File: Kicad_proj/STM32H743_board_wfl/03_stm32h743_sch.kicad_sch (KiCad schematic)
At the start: 1 part, among them U1 STM32H743VITx

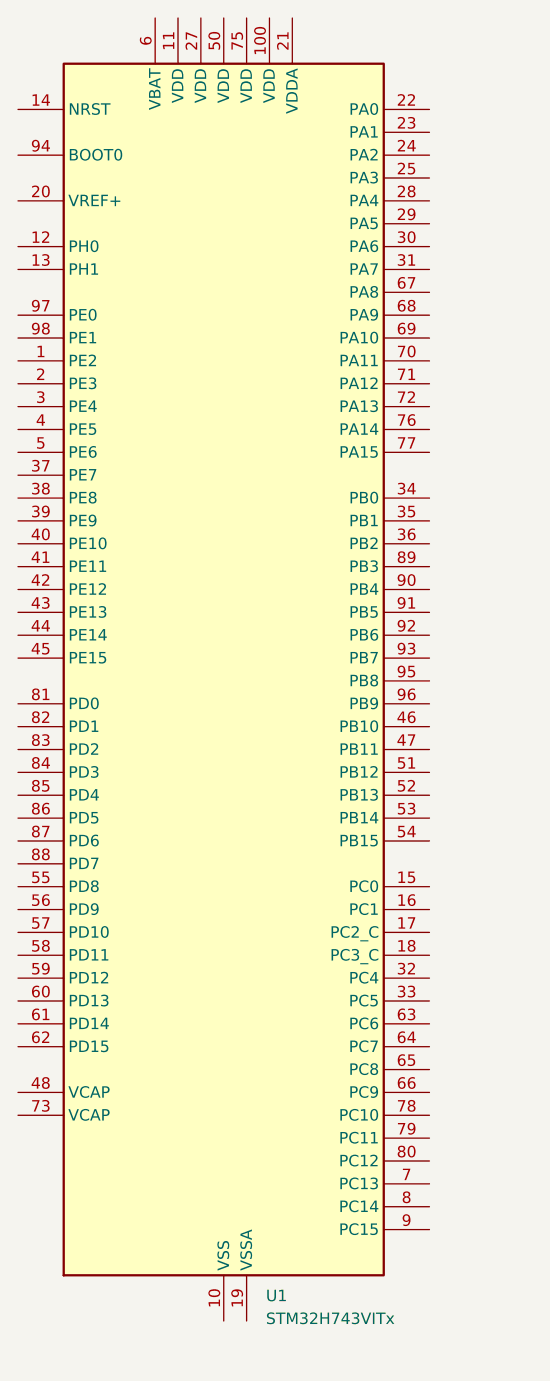
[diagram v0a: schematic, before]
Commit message: v0.3 uzupelniony prebom + placement BMI088 na sch
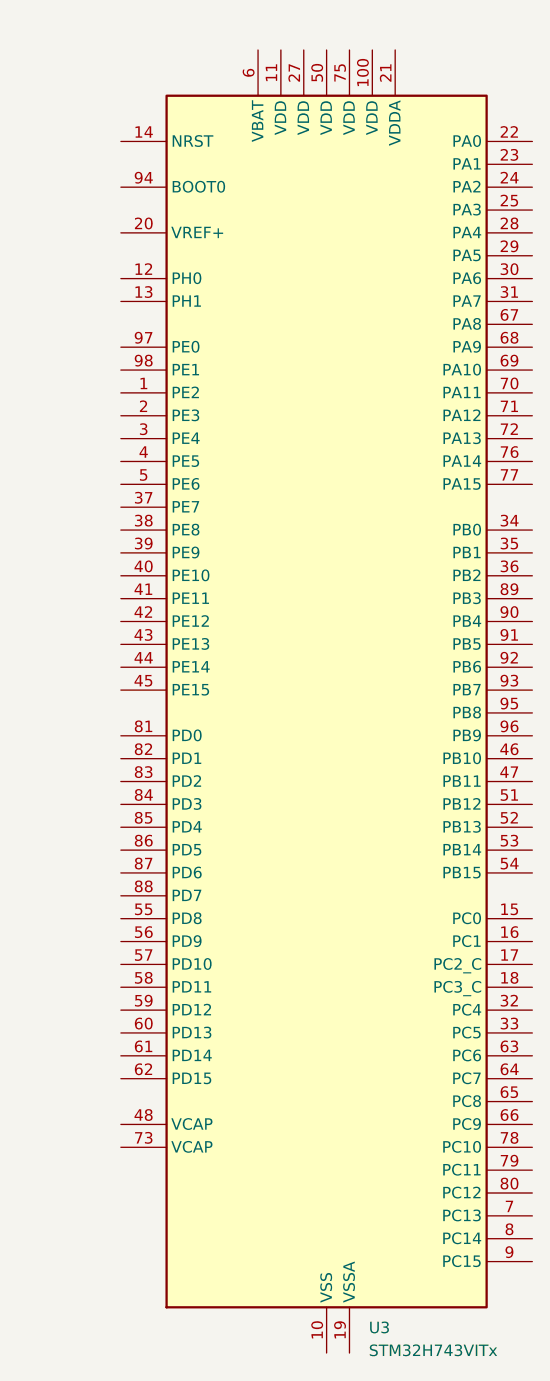
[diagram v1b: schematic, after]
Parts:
- renumbered U1 to U3
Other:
- moved on the sheet: U3
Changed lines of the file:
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@@
 	(symbol
 		(lib_id "MCU_ST_STM32H7:STM32H743VITx")
-		(at 214.884 132.588 0)
+		(at 226.314 136.144 0)
 		(unit 1)
 		(body_style 1)
@@
 		(dnp no)
 		(fields_autoplaced yes)
-		(property "Reference" "U1"
-			(at 219.5673 200.914 0)
+		(property "Reference" "U3"
+			(at 230.9973 204.47 0)
 			(show_name no)
 			(do_not_autoplace no)
@@
 		)
 		(property "Value" "STM32H743VITx"
-			(at 219.5673 203.454 0)
+			(at 230.9973 207.01 0)
 			(show_name no)
 			(do_not_autoplace no)
@@
 		)
 		(property "Footprint" "Package_QFP:LQFP-100_14x14mm_P0.5mm"
-			(at 197.104 198.628 0)
+			(at 208.534 202.184 0)
 			(hide yes)
 			(show_name no)
@@
 		)
 		(property "Datasheet" "https://www.st.com/resource/en/datasheet/stm32h743vi.pdf"
-			(at 214.884 132.588 0)
+			(at 226.314 136.144 0)
 			(hide yes)
 			(show_name no)
@@
 		)
 		(property "Description" "STMicroelectronics Arm Cortex-M7 MCU, 2048KB flash, 1024KB RAM, 480 MHz, 1.71-3.6V, 82 GPIO, LQFP100"
-			(at 214.884 132.588 0)
+			(at 226.314 136.144 0)
 			(hide yes)
 			(show_name no)
@@
 			(project "STM32H743_board_wfl"
 				(path "/3ffbaf01-8fe7-4f96-b685-21b9df9d548a/d99da23c-42db-4338-87a0-b38c4540e099"
-					(reference "U1")
+					(reference "U3")
 					(unit 1)
 				)

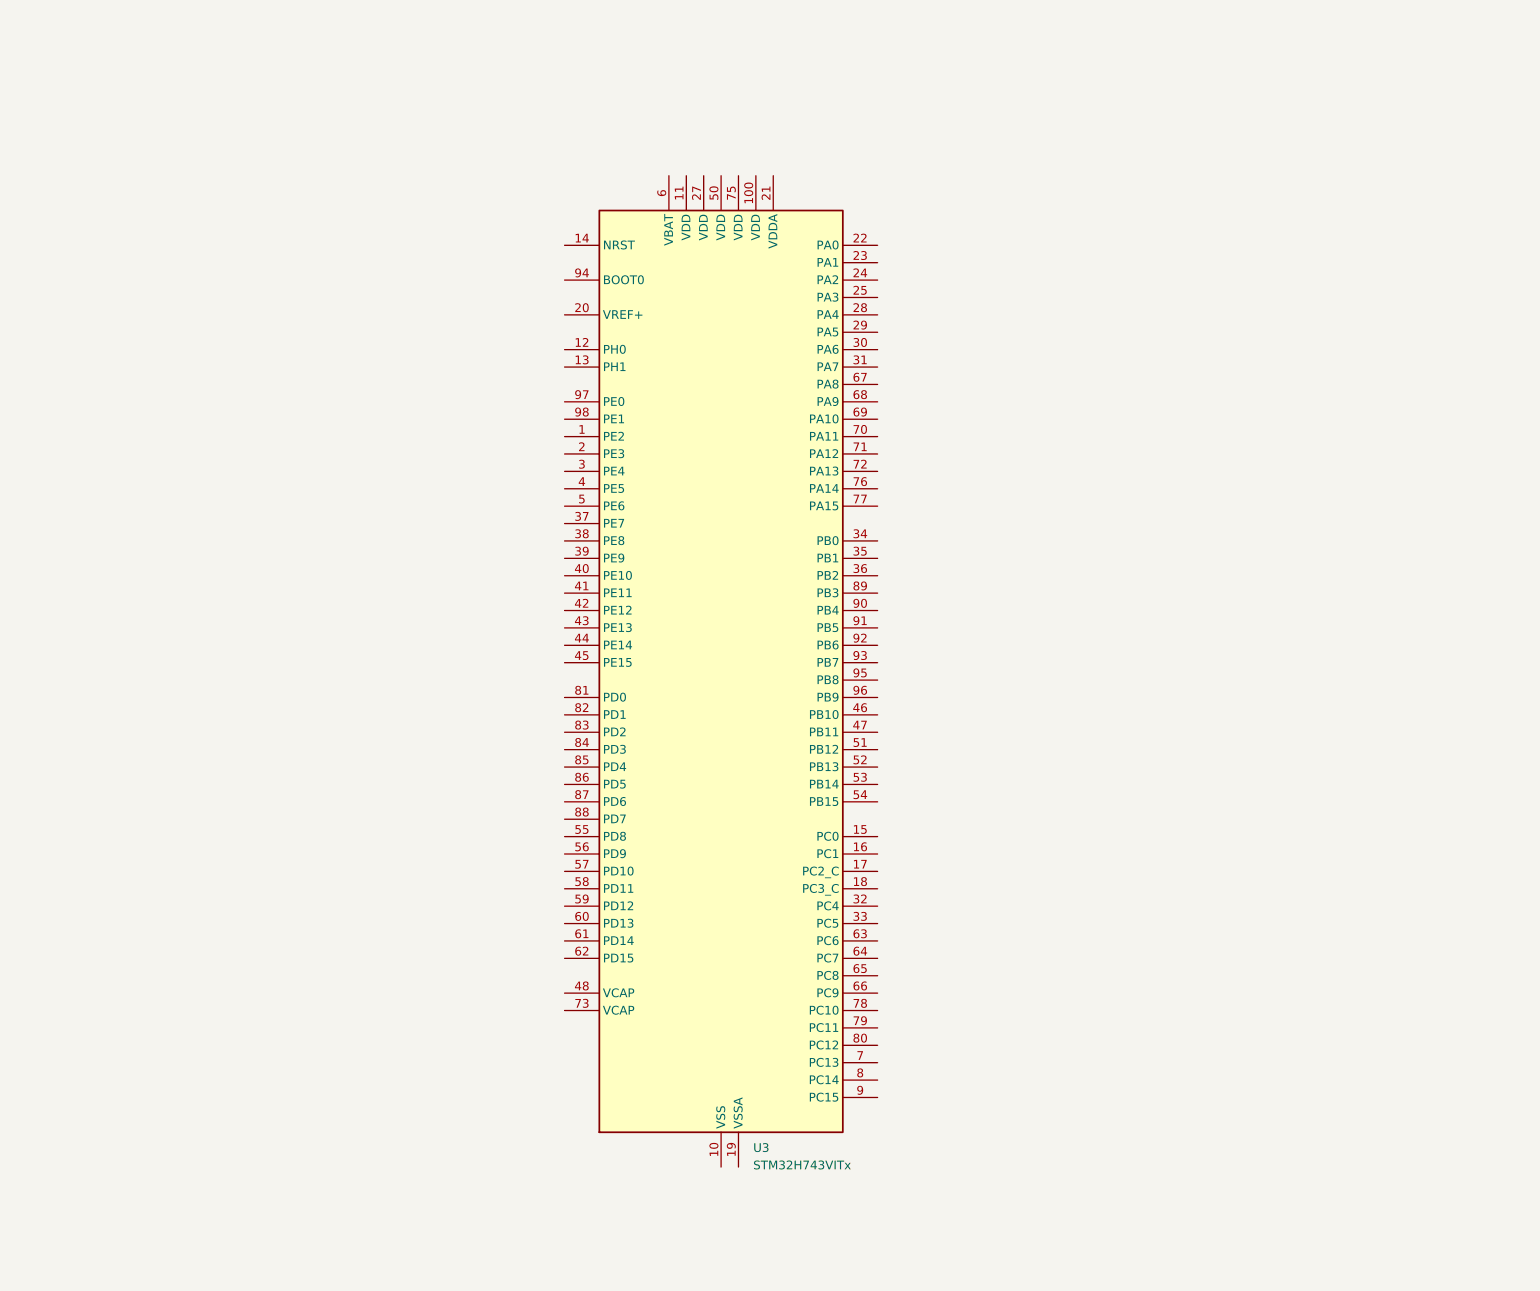
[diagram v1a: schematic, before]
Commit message: v0.4c stm
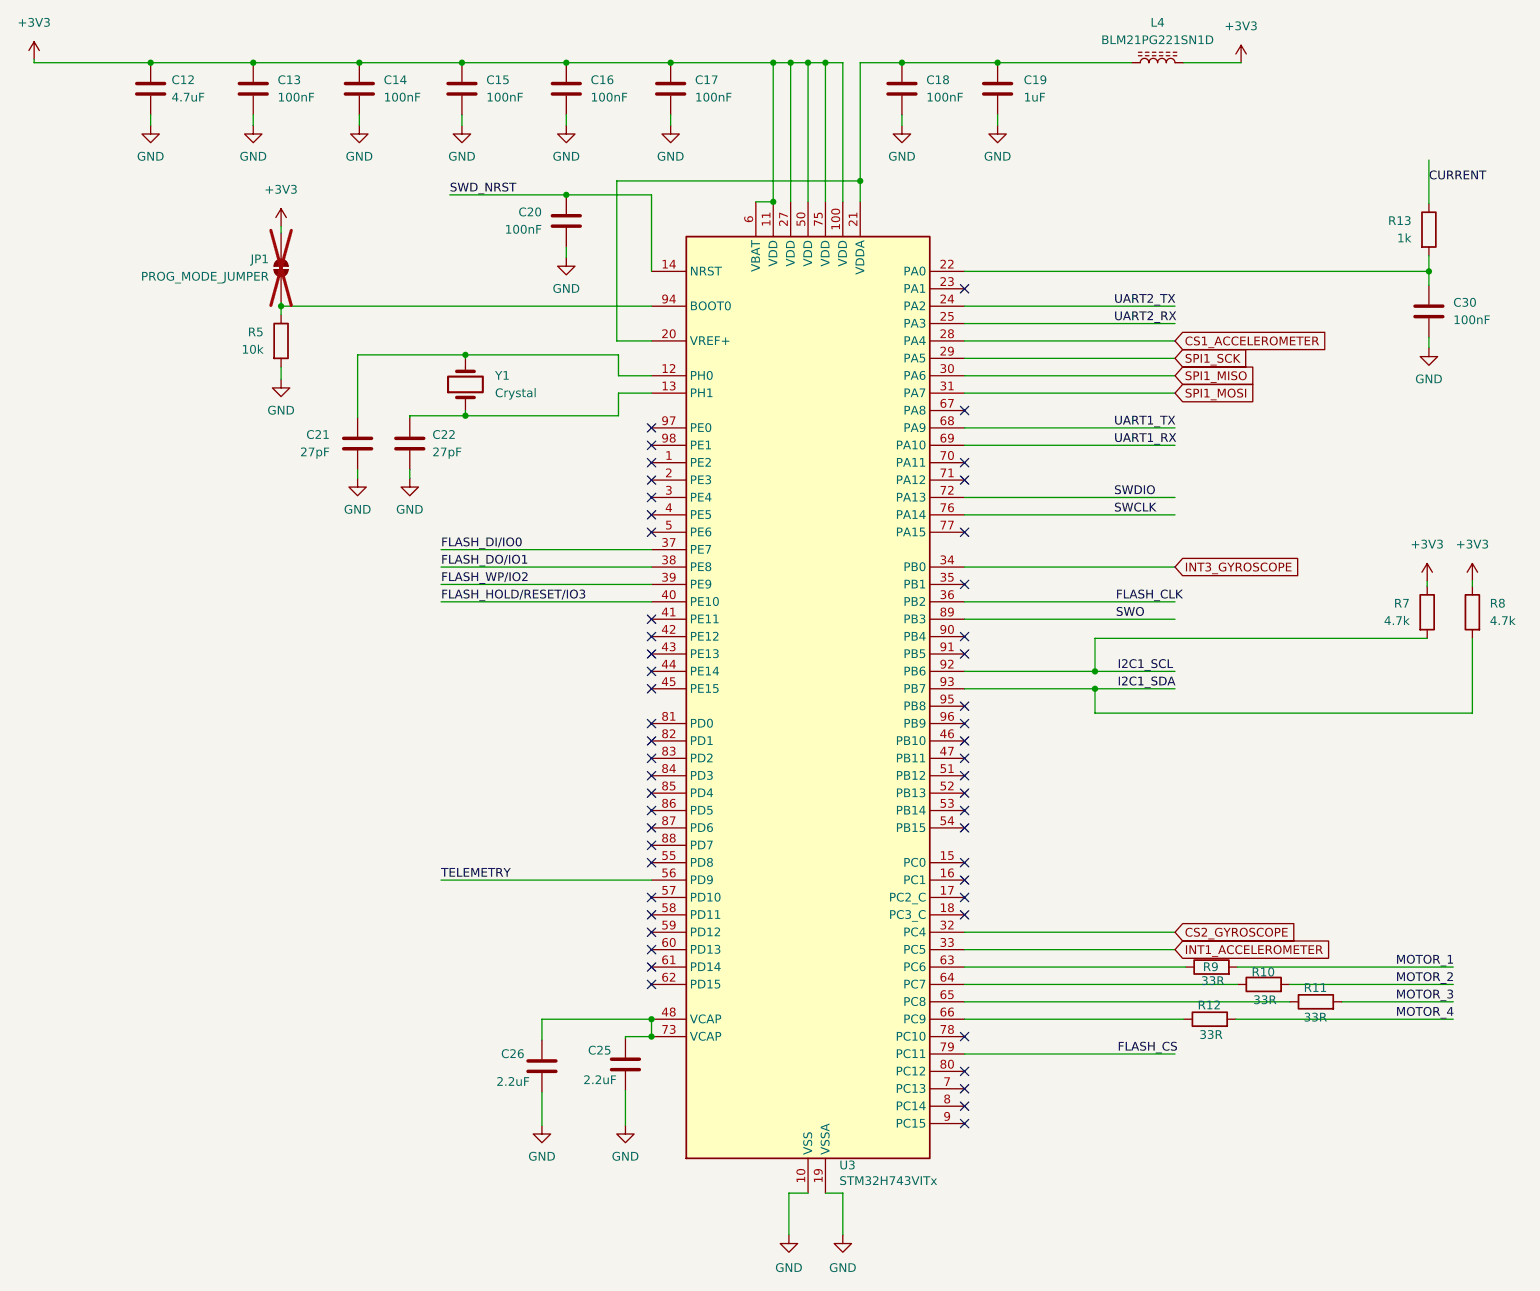
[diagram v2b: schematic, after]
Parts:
- added C12: 4.7uF, Capacitor_SMD:C_0603_1608Metric, symbol Device:C
- added C13, C14, C15, C16, C17, C18, C20, C30: 100nF, Capacitor_SMD:C_0402_1005Metric, symbol Device:C
- added C19: 1uF, Capacitor_SMD:C_0603_1608Metric, symbol Device:C
- added C21, C22: 27pF, Capacitor_SMD:C_0402_1005Metric, symbol Device:C
- added C25, C26: 2.2uF, Capacitor_SMD:C_0603_1608Metric, symbol Device:C
- added JP1: PROG_MODE_JUMPER, Resistor_SMD:R_01005_0402Metric, symbol Jumper:SolderJumper_2_Open
- added L4: BLM21PG221SN1D, Inductor_SMD:L_0805_2012Metric, symbol Device:L_Ferrite
- added R10, R11, R12, R9: 33R, Resistor_SMD:R_01005_0402Metric, symbol Device:R
- added R13: 1k, Resistor_SMD:R_01005_0402Metric, symbol Device:R
- added R5: 10k, Resistor_SMD:R_01005_0402Metric, symbol Device:R
- added R7, R8: 4.7k, Resistor_SMD:R_01005_0402Metric, symbol Device:R
- added Y1: Crystal, Crystal:Crystal_SMD_Abracon_ABM3-2Pin_5.0x3.2mm, symbol Device:Crystal
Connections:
- net GND: now reaches U3.10 (VSS), U3.26 (VSS), U3.49 (VSS), U3.74 (VSS), U3.99 (VSS)
- net GND: now also U3.19 (VSSA), C12.2, C13.2, C14.2, C15.2, C16.2, C17.2, C18.2, C19.2, C20.2, C21.2, C22.2, C25.2, C26.2, C30.2, R5.2
- net +3V3: now reaches U3.100 (VDD)
- net +3V3: now also U3.11 (VDD), U3.27 (VDD), U3.50 (VDD), U3.6 (VBAT), U3.75 (VDD), C12.1, C13.1, C14.1, C15.1, C16.1, C17.1, JP1.2 (B), L4.2, R7.1, R8.1
- net at U3.12 (PH0): now also C21.1, Y1.2
- net at U3.13 (PH1): now also C22.1, Y1.1
- net SWD_NRST: now reaches U3.14 (NRST)
- net SWD_NRST: now also C20.1
- net at U3.20 (VREF+): now also U3.21 (VDDA), C18.1, C19.1, L4.1
- net at U3.22 (PA0): now also C30.1, R13.2
- net UART2_TX: now reaches U3.24 (PA2)
- net UART2_RX: now reaches U3.25 (PA3)
- net CS1_ACCELEROMETER: now reaches U3.28 (PA4)
- net SPI1_SCK: now reaches U3.29 (PA5)
- net SPI1_MISO: now reaches U3.30 (PA6)
- net SPI1_MOSI: now reaches U3.31 (PA7)
- net CS2_GYROSCOPE: now reaches U3.32 (PC4)
- net INT1_ACCELEROMETER: now reaches U3.33 (PC5)
- net INT3_GYROSCOPE: now reaches U3.34 (PB0)
- net FLASH_CLK: now reaches U3.36 (PB2)
- net FLASH_DI/IO0: now reaches U3.37 (PE7)
- net FLASH_DO/IO1: now reaches U3.38 (PE8)
- net FLASH_WP/IO2: now reaches U3.39 (PE9)
- net FLASH_HOLD/RESET/IO3: now reaches U3.40 (PE10)
- net at U3.48 (VCAP): now also U3.73 (VCAP), C25.1, C26.1
- net TELEMETRY: now reaches U3.56 (PD9)
- net at U3.63 (PC6): now also R9.1
- net at U3.64 (PC7): now also R10.1
- net at U3.65 (PC8): now also R11.1
- net at U3.66 (PC9): now also R12.1
- net UART1_TX: now reaches U3.68 (PA9)
- net UART1_RX: now reaches U3.69 (PA10)
- net SWDIO: now reaches U3.72 (PA13)
- net SWCLK: now reaches U3.76 (PA14)
- net FLASH_CS: now reaches U3.79 (PC11)
- net SWO: now reaches U3.89 (PB3)
- net I2C1_SCL: now reaches U3.92 (PB6)
- net I2C1_SCL: now also R7.2
- net I2C1_SDA: now reaches U3.93 (PB7)
- net I2C1_SDA: now also R8.2
- net at U3.94 (BOOT0): now also JP1.1 (A), R5.1
- new net CURRENT: R13.1
- new net MOTOR_1: R9.2
- new net MOTOR_2: R10.2
- new net MOTOR_3: R11.2
- new net MOTOR_4: R12.2
- no-connect marks 0 -> 52
